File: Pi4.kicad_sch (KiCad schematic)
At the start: 3 parts, among them U601 RASPBERRY_PI_4B_4GB

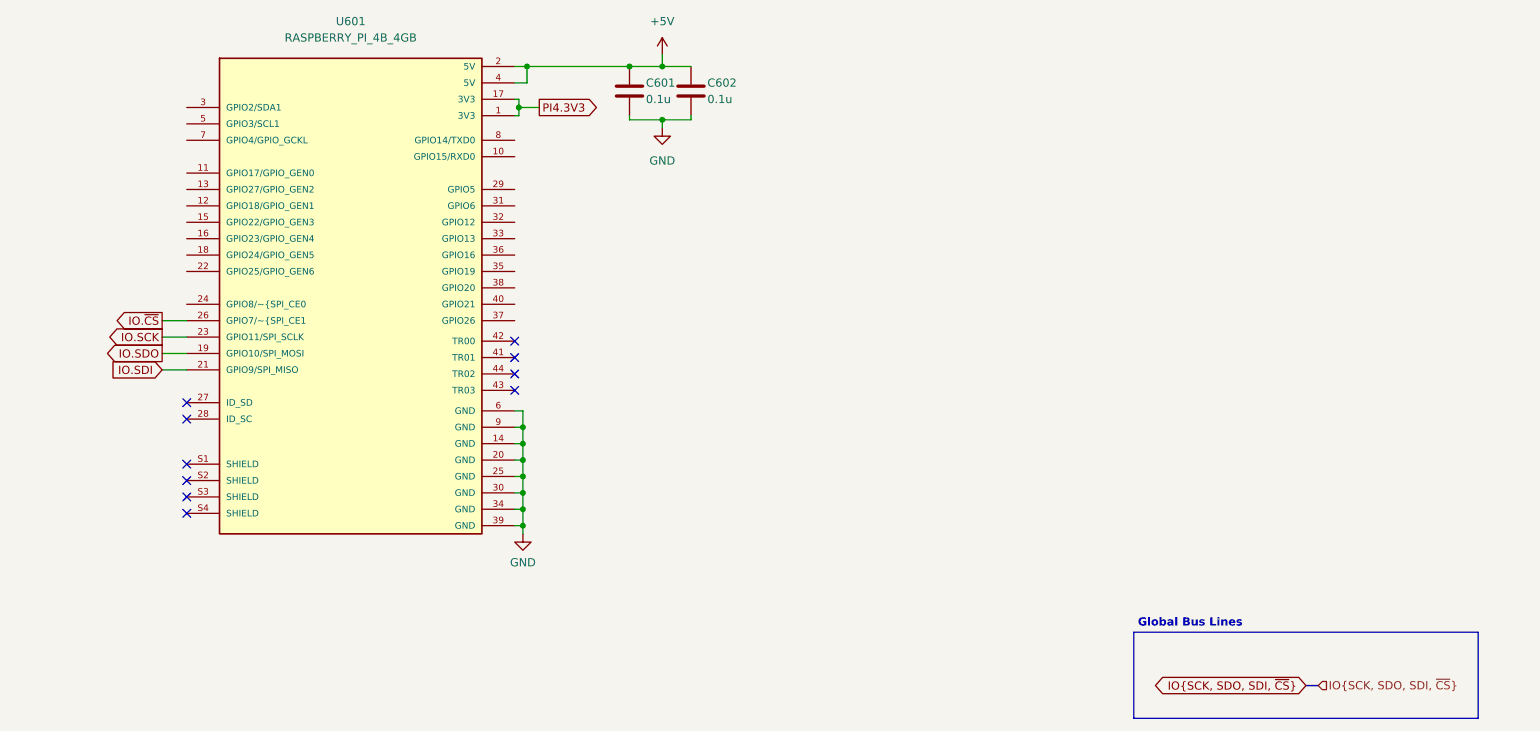
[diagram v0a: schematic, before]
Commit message: Update 1
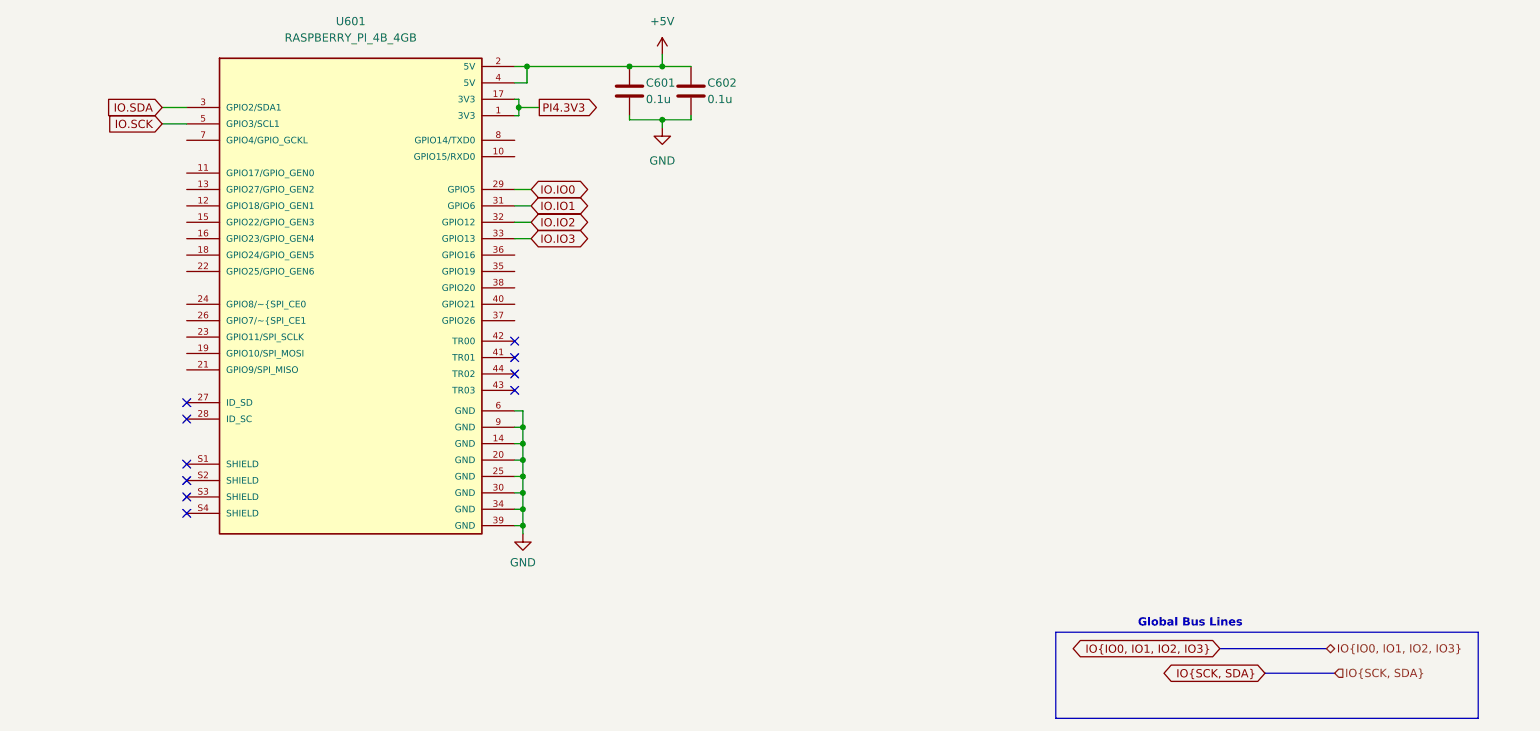
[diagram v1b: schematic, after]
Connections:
- net IO.SCK: now also U601.5 (GPIO3/SCL1); no longer U601.23 (GPIO11/SPI_SCLK)
- net IO.IO0: now reaches U601.29 (GPIO5)
- net IO.SDA: now reaches U601.3 (GPIO2/SDA1)
- net IO.IO1: now reaches U601.31 (GPIO6)
- net IO.IO2: now reaches U601.32 (GPIO12)
- net IO.IO3: now reaches U601.33 (GPIO13)
- net IO.SDI: no longer names the net of U601.21 (GPIO9/SPI_MISO)
- net IO.SDO: no longer names the net of U601.19 (GPIO10/SPI_MOSI)
- net IO.~{CS}: no longer names the net of U601.26 (GPIO7/~{SPI_CE1~{})
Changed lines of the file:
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@@
+    (stroke (width 0) (type default) (color 0 0 0 0))
+  )
+  (wire (pts (xy 74.93 69.215) (xy 78.74 69.215))
     (stroke (width 0) (type default) (color 0 0 0 0))
   )
@@
     (stroke (width 0) (type default) (color 0 0 0 0))
   )
-  (polyline (pts (xy 225.425 150.495) (xy 225.425 163.83))
+  (polyline (pts (xy 213.36 150.495) (xy 213.36 163.83))
     (stroke (width 0) (type default) (color 0 0 0 0))
   )
@@
   )
   (wire (pts (xy 147.32 71.12) (xy 152.4 71.12))
+    (stroke (width 0) (type default) (color 0 0 0 0))
+  )
+  (wire (pts (xy 129.54 81.915) (xy 132.08 81.915))
     (stroke (width 0) (type default) (color 0 0 0 0))
   )
@@
     (stroke (width 0) (type default) (color 0 0 0 0))
   )
-  (wire (pts (xy 74.93 102.235) (xy 78.74 102.235))
+  (wire (pts (xy 129.54 86.995) (xy 132.08 86.995))
     (stroke (width 0) (type default) (color 0 0 0 0))
   )
-  (polyline (pts (xy 225.425 163.83) (xy 278.765 163.83))
+  (polyline (pts (xy 213.36 163.83) (xy 278.765 163.83))
     (stroke (width 0) (type default) (color 0 0 0 0))
   )
@@
     (stroke (width 0) (type default) (color 0 0 0 0))
   )
+  (wire (pts (xy 129.54 89.535) (xy 132.08 89.535))
+    (stroke (width 0) (type default) (color 0 0 0 0))
+  )
   (wire (pts (xy 156.845 71.12) (xy 156.845 70.485))
     (stroke (width 0) (type default) (color 0 0 0 0))
@@
     (stroke (width 0) (type default) (color 0 0 0 0))
   )
+  (wire (pts (xy 129.54 84.455) (xy 132.08 84.455))
+    (stroke (width 0) (type default) (color 0 0 0 0))
+  )
   (wire (pts (xy 130.175 69.215) (xy 133.35 69.215))
     (stroke (width 0) (type default) (color 0 0 0 0))
   )
   (wire (pts (xy 129.54 67.945) (xy 130.175 67.945))
+    (stroke (width 0) (type default) (color 0 0 0 0))
+  )
+  (bus (pts (xy 245.745 156.845) (xy 256.54 156.845))
     (stroke (width 0) (type default) (color 0 0 0 0))
   )
@@
     (stroke (width 0) (type default) (color 0 0 0 0))
   )
-  (bus (pts (xy 252.095 158.75) (xy 254 158.75))
-    (stroke (width 0) (type default) (color 0 0 0 0))
-  )
   (wire (pts (xy 129.54 62.865) (xy 131.445 62.865))
     (stroke (width 0) (type default) (color 0 0 0 0))
@@
     (stroke (width 0) (type default) (color 0 0 0 0))
   )
-  (wire (pts (xy 74.93 109.855) (xy 78.74 109.855))
-    (stroke (width 0) (type default) (color 0 0 0 0))
-  )
   (wire (pts (xy 130.81 121.285) (xy 130.81 118.745))
     (stroke (width 0) (type default) (color 0 0 0 0))
@@
     (stroke (width 0) (type default) (color 0 0 0 0))
   )
-  (wire (pts (xy 74.93 107.315) (xy 78.74 107.315))
+  (wire (pts (xy 74.93 71.755) (xy 78.74 71.755))
     (stroke (width 0) (type default) (color 0 0 0 0))
   )
@@
     (stroke (width 0) (type default) (color 0 0 0 0))
   )
-  (wire (pts (xy 74.93 104.775) (xy 78.74 104.775))
+  (bus (pts (xy 238.76 153.035) (xy 255.27 153.035))
     (stroke (width 0) (type default) (color 0 0 0 0))
   )
@@
     (stroke (width 0) (type default) (color 0 0 0 0))
   )
-  (polyline (pts (xy 278.765 150.495) (xy 225.425 150.495))
+  (polyline (pts (xy 278.765 150.495) (xy 213.36 150.495))
     (stroke (width 0) (type default) (color 0 0 0 0))
   )
@@
     (effects (font (size 1.27 1.27) (thickness 0.254) bold) (justify left bottom))
   )
-  (global_label "IO.~{CS}" (shape output) (at 74.93 102.235 180) (fields_autoplaced)
+  (global_label "IO.SCK" (shape input) (at 74.93 71.755 180) (fields_autoplaced)
     (effects (font (size 1.27 1.27)) (justify right))
-    (property "Intersheet References" "${INTERSHEET_REFS}" (id 0) (at 67.4974 102.1556 0)
+    (property "Intersheet References" "${INTERSHEET_REFS}" (id 0) (at 66.2274 71.6756 0)
       (effects (font (size 1.27 1.27)) (justify right) hide)
     )
   )
-  (global_label "IO.SDO" (shape output) (at 74.93 107.315 180) (fields_autoplaced)
-    (effects (font (size 1.27 1.27)) (justify right))
-    (property "Intersheet References" "${INTERSHEET_REFS}" (id 0) (at 66.1669 107.2356 0)
-      (effects (font (size 1.27 1.27)) (justify right) hide)
+  (global_label "IO.IO0" (shape bidirectional) (at 132.08 81.915 0) (fields_autoplaced)
+    (effects (font (size 1.27 1.27)) (justify left))
+    (property "Intersheet References" "${INTERSHEET_REFS}" (id 0) (at 140.1779 81.8356 0)
+      (effects (font (size 1.27 1.27)) (justify left) hide)
     )
   )
@@
     )
   )
-  (global_label "IO{SCK, SDO, SDI, ~{CS}}" (shape bidirectional) (at 252.095 158.75 180) (fields_autoplaced)
+  (global_label "IO.IO3" (shape bidirectional) (at 132.08 89.535 0) (fields_autoplaced)
+    (effects (font (size 1.27 1.27)) (justify left))
+    (property "Intersheet References" "${INTERSHEET_REFS}" (id 0) (at 140.1779 89.4556 0)
+      (effects (font (size 1.27 1.27)) (justify left) hide)
+    )
+  )
+  (global_label "IO{IO0, IO1, IO2, IO3}" (shape bidirectional) (at 238.76 153.035 180) (fields_autoplaced)
     (effects (font (size 1.27 1.27)) (justify right))
-    (property "Intersheet References" "${INTERSHEET_REFS}" (id 0) (at 228.2129 158.6706 0)
+    (property "Intersheet References" "${INTERSHEET_REFS}" (id 0) (at 215.4221 152.9556 0)
       (effects (font (size 1.27 1.27)) (justify right) hide)
     )
   )
-  (global_label "IO.SCK" (shape output) (at 74.93 104.775 180) (fields_autoplaced)
+  (global_label "IO.IO1" (shape bidirectional) (at 132.08 84.455 0) (fields_autoplaced)
+    (effects (font (size 1.27 1.27)) (justify left))
+    (property "Intersheet References" "${INTERSHEET_REFS}" (id 0) (at 140.1779 84.3756 0)
+      (effects (font (size 1.27 1.27)) (justify left) hide)
+    )
+  )
+  (global_label "IO.IO2" (shape bidirectional) (at 132.08 86.995 0) (fields_autoplaced)
+    (effects (font (size 1.27 1.27)) (justify left))
+    (property "Intersheet References" "${INTERSHEET_REFS}" (id 0) (at 140.1779 86.9156 0)
+      (effects (font (size 1.27 1.27)) (justify left) hide)
+    )
+  )
+  (global_label "IO.SDA" (shape input) (at 74.93 69.215 180) (fields_autoplaced)
     (effects (font (size 1.27 1.27)) (justify right))
-    (property "Intersheet References" "${INTERSHEET_REFS}" (id 0) (at 66.2274 104.6956 0)
+    (property "Intersheet References" "${INTERSHEET_REFS}" (id 0) (at 66.4088 69.1356 0)
       (effects (font (size 1.27 1.27)) (justify right) hide)
     )
   )
-  (global_label "IO.SDI" (shape input) (at 74.93 109.855 180) (fields_autoplaced)
+  (global_label "IO{SCK, SDA}" (shape bidirectional) (at 245.745 156.845 180) (fields_autoplaced)
     (effects (font (size 1.27 1.27)) (justify right))
-    (property "Intersheet References" "${INTERSHEET_REFS}" (id 0) (at 66.8926 109.7756 0)
+    (property "Intersheet References" "${INTERSHEET_REFS}" (id 0) (at 230.8133 156.7656 0)
       (effects (font (size 1.27 1.27)) (justify right) hide)
     )
   )
-  (hierarchical_label "IO{SCK, SDO, SDI, ~{CS}}" (shape input) (at 254 158.75 0)
+  (hierarchical_label "IO{IO0, IO1, IO2, IO3}" (shape bidirectional) (at 255.27 153.035 0)
     (effects (font (size 1.27 1.27)) (justify left))
   )
+  (hierarchical_label "IO{SCK, SDA}" (shape input) (at 256.54 156.845 0)
+    (effects (font (size 1.27 1.27)) (justify left))
+  )

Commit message: Update 2nd iteration
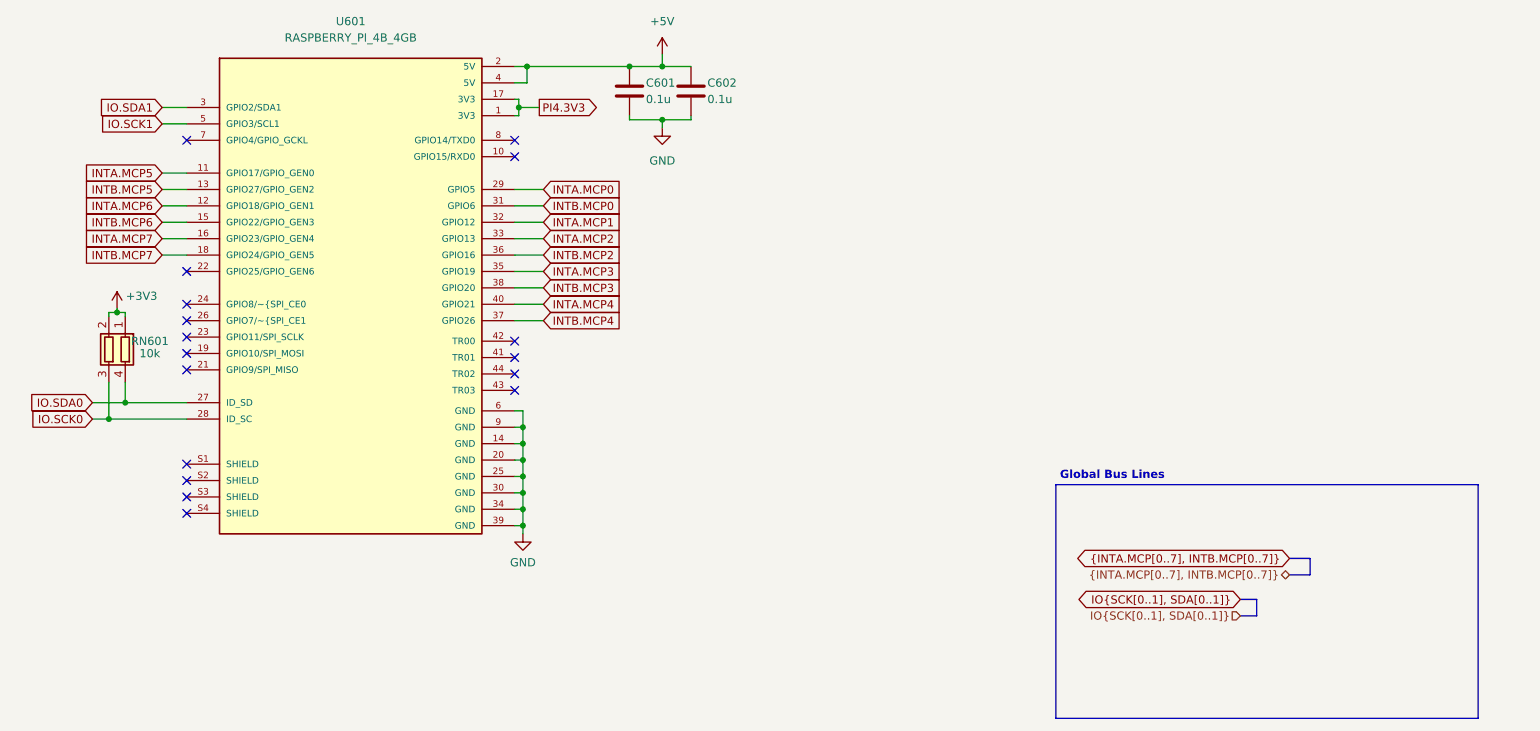
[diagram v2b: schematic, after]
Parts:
- added RN601: 10k, Resistor_SMD:R_Array_Convex_2x0402, symbol Device:R_Pack02
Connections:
- net INTA.MCP5: now reaches U601.11 (GPIO17/GPIO_GEN0)
- net INTA.MCP6: now reaches U601.12 (GPIO18/GPIO_GEN1)
- net INTB.MCP5: now reaches U601.13 (GPIO27/GPIO_GEN2)
- net INTB.MCP6: now reaches U601.15 (GPIO22/GPIO_GEN3)
- net INTA.MCP7: now reaches U601.16 (GPIO23/GPIO_GEN4)
- net INTB.MCP7: now reaches U601.18 (GPIO24/GPIO_GEN5)
- net IO.SDA0: now reaches U601.27 (ID_SD)
- net IO.SDA0: now also RN601.4 (R1.2)
- net IO.SCK0: now reaches U601.28 (ID_SC)
- net IO.SCK0: now also RN601.3 (R2.2)
- net INTA.MCP3: now reaches U601.35 (GPIO19)
- net INTB.MCP2: now reaches U601.36 (GPIO16)
- net INTB.MCP4: now reaches U601.37 (GPIO26)
- net INTB.MCP3: now reaches U601.38 (GPIO20)
- net INTA.MCP4: now reaches U601.40 (GPIO21)
- net IO.IO0 renamed INTA.MCP0
- net IO.IO1 renamed INTB.MCP0
- net IO.IO2 renamed INTA.MCP1
- net IO.IO3 renamed INTA.MCP2
- net IO.SCK renamed IO.SCK1
- net IO.SDA renamed IO.SDA1
- new net +3V3: RN601.1 (R1.1), RN601.2 (R2.1)
- no-connect marks 10 -> 17
